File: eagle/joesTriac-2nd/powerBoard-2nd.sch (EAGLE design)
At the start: 17 parts, among them IC1 7809, IC2 7805, IC3 7909, J1 XF2E-0815-1, J2 XF2E-0815-1

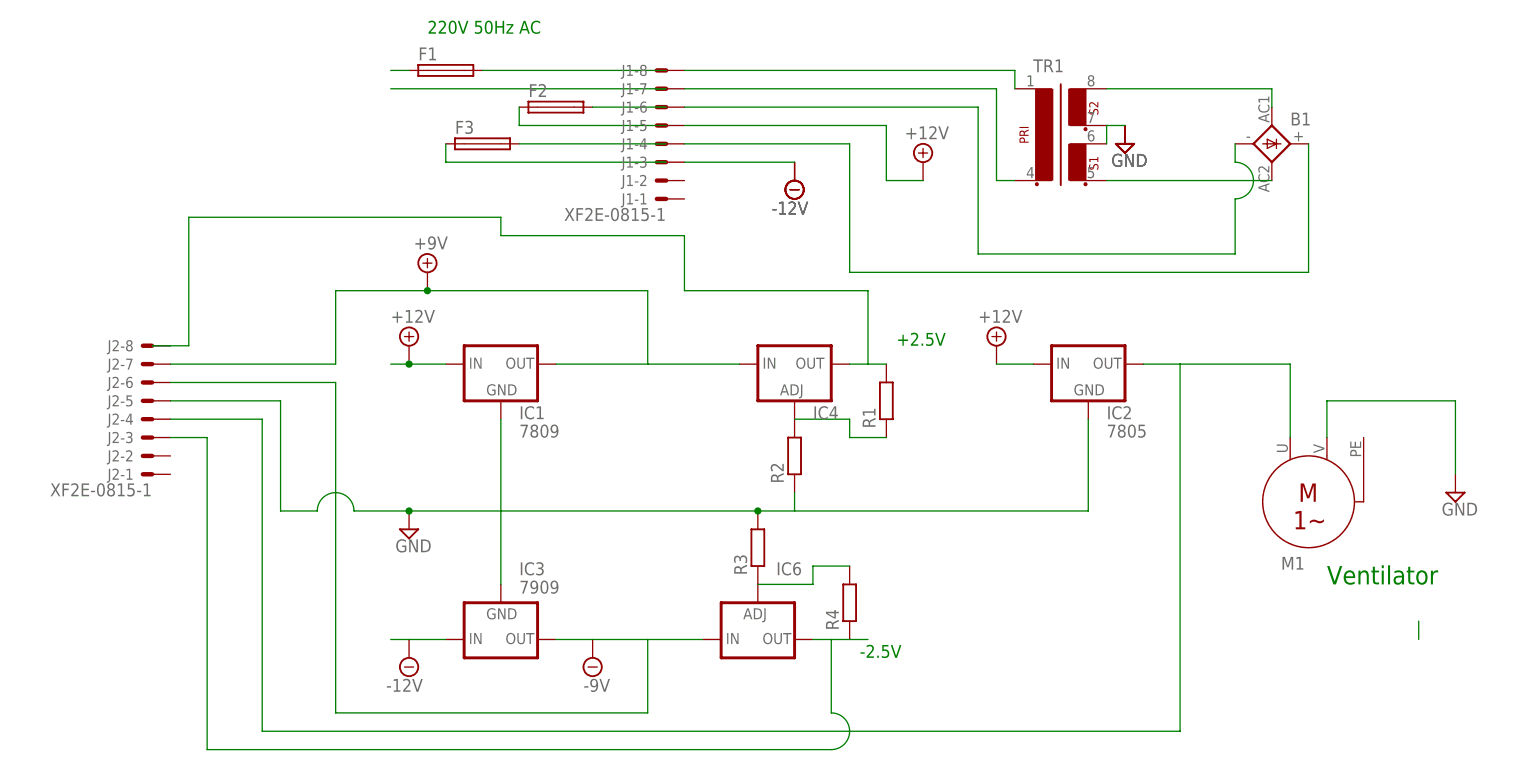
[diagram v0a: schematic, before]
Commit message: reg save
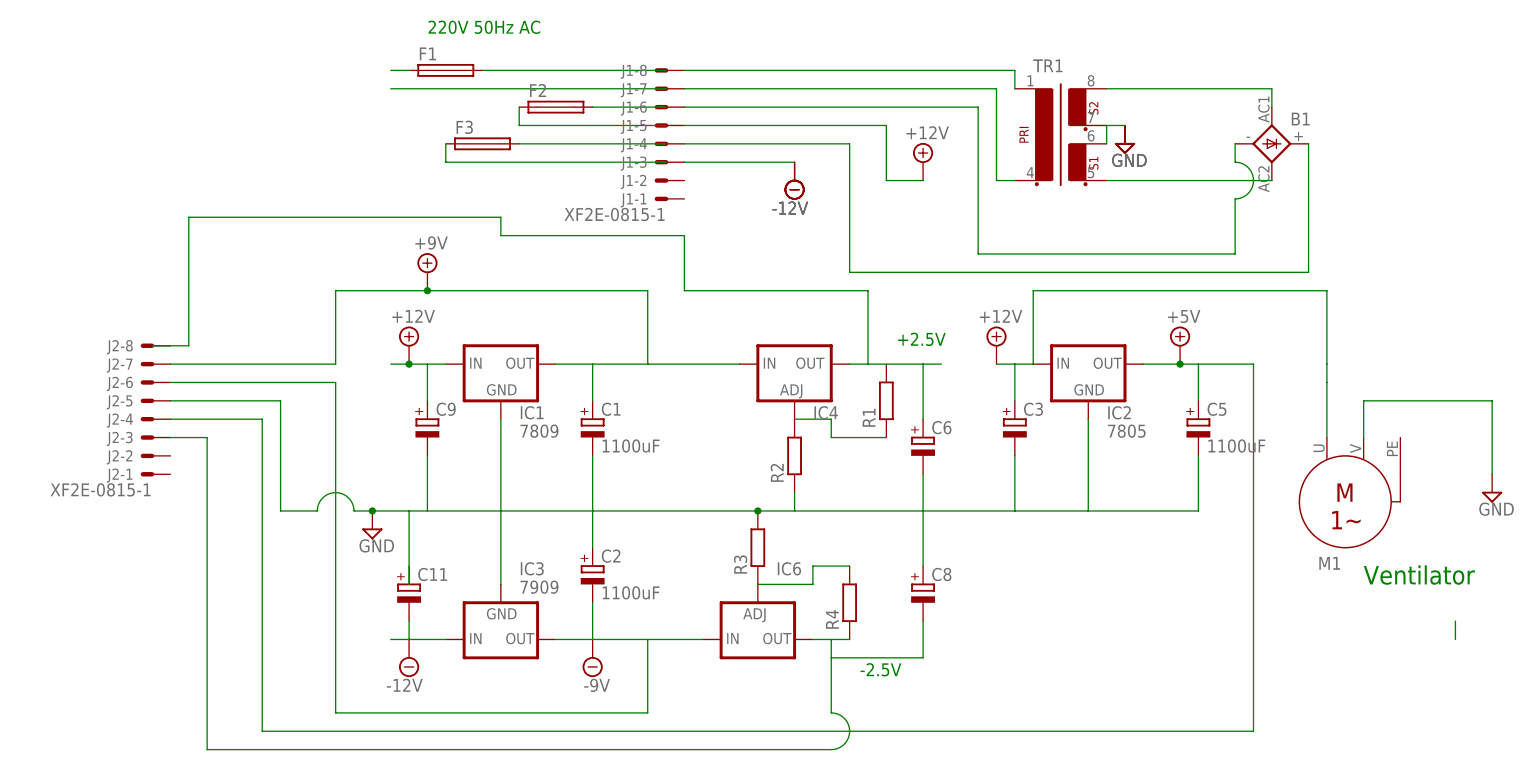
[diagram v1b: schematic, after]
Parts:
- added C1, C2, C5: 1100uF, resistor:CPOL-EUE22-6AXIAL
- added C11, C3, C6, C8, C9: (no value), resistor:CPOL-EUE22-6AXIAL
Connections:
- removed net N$10: IC2.OUT, J2-4.MS, M1.U
- new net +5V: C5.+, IC2.OUT, J2-4.MS
- net +12V: now also C3.+, C9.+, M1.U
- net +9V: now also C1.+
- net -12V: now also C11.-
- net -9V: now also C2.-
- net GND: now also C1.-, C2.+, C3.-, C5.-, C6.-, C8.+, C9.-
- net N$21: now also C8.-, R4.1
- net N$23: now also C6.+
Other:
- moved on the sheet: M1
